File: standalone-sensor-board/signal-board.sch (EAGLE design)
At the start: 26 parts, among them U1 CD4051BE

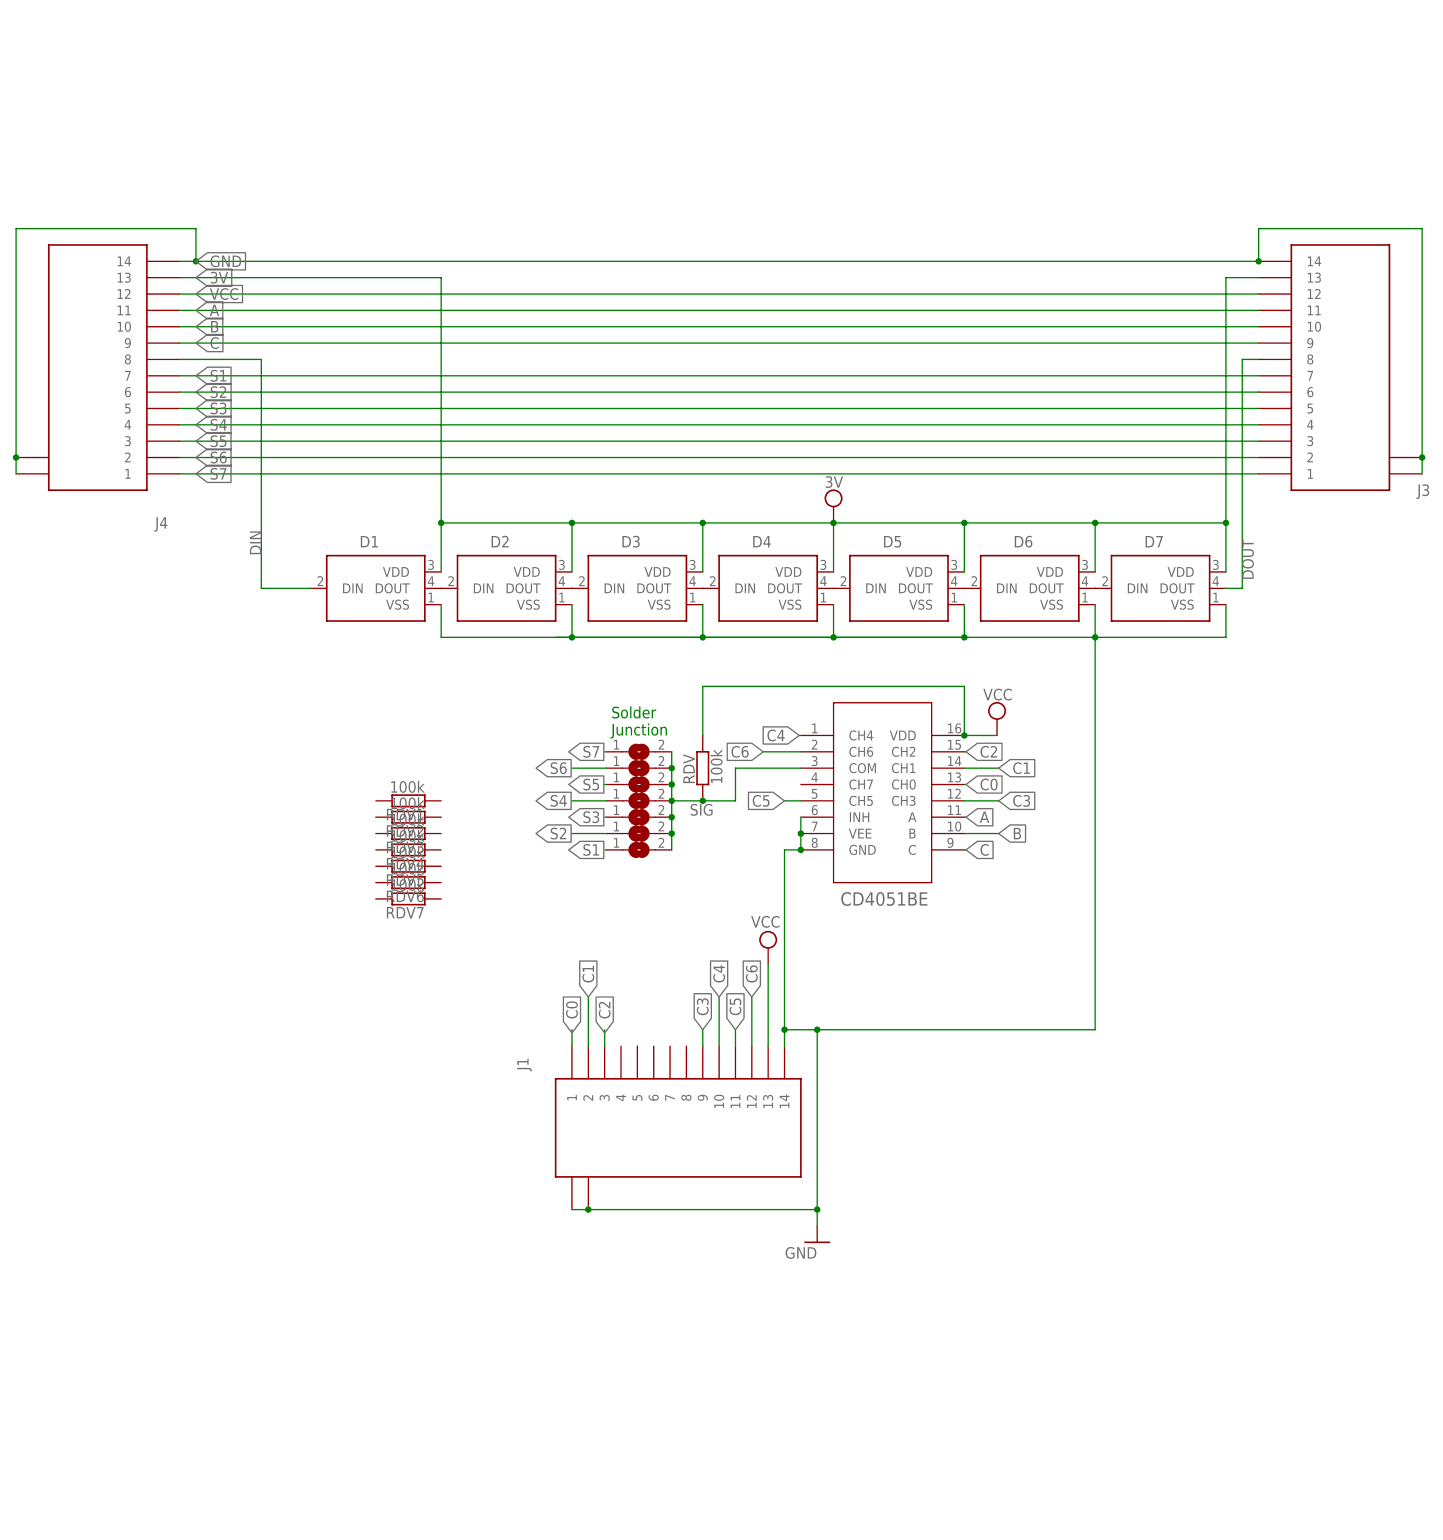
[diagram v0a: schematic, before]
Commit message: set rdvs
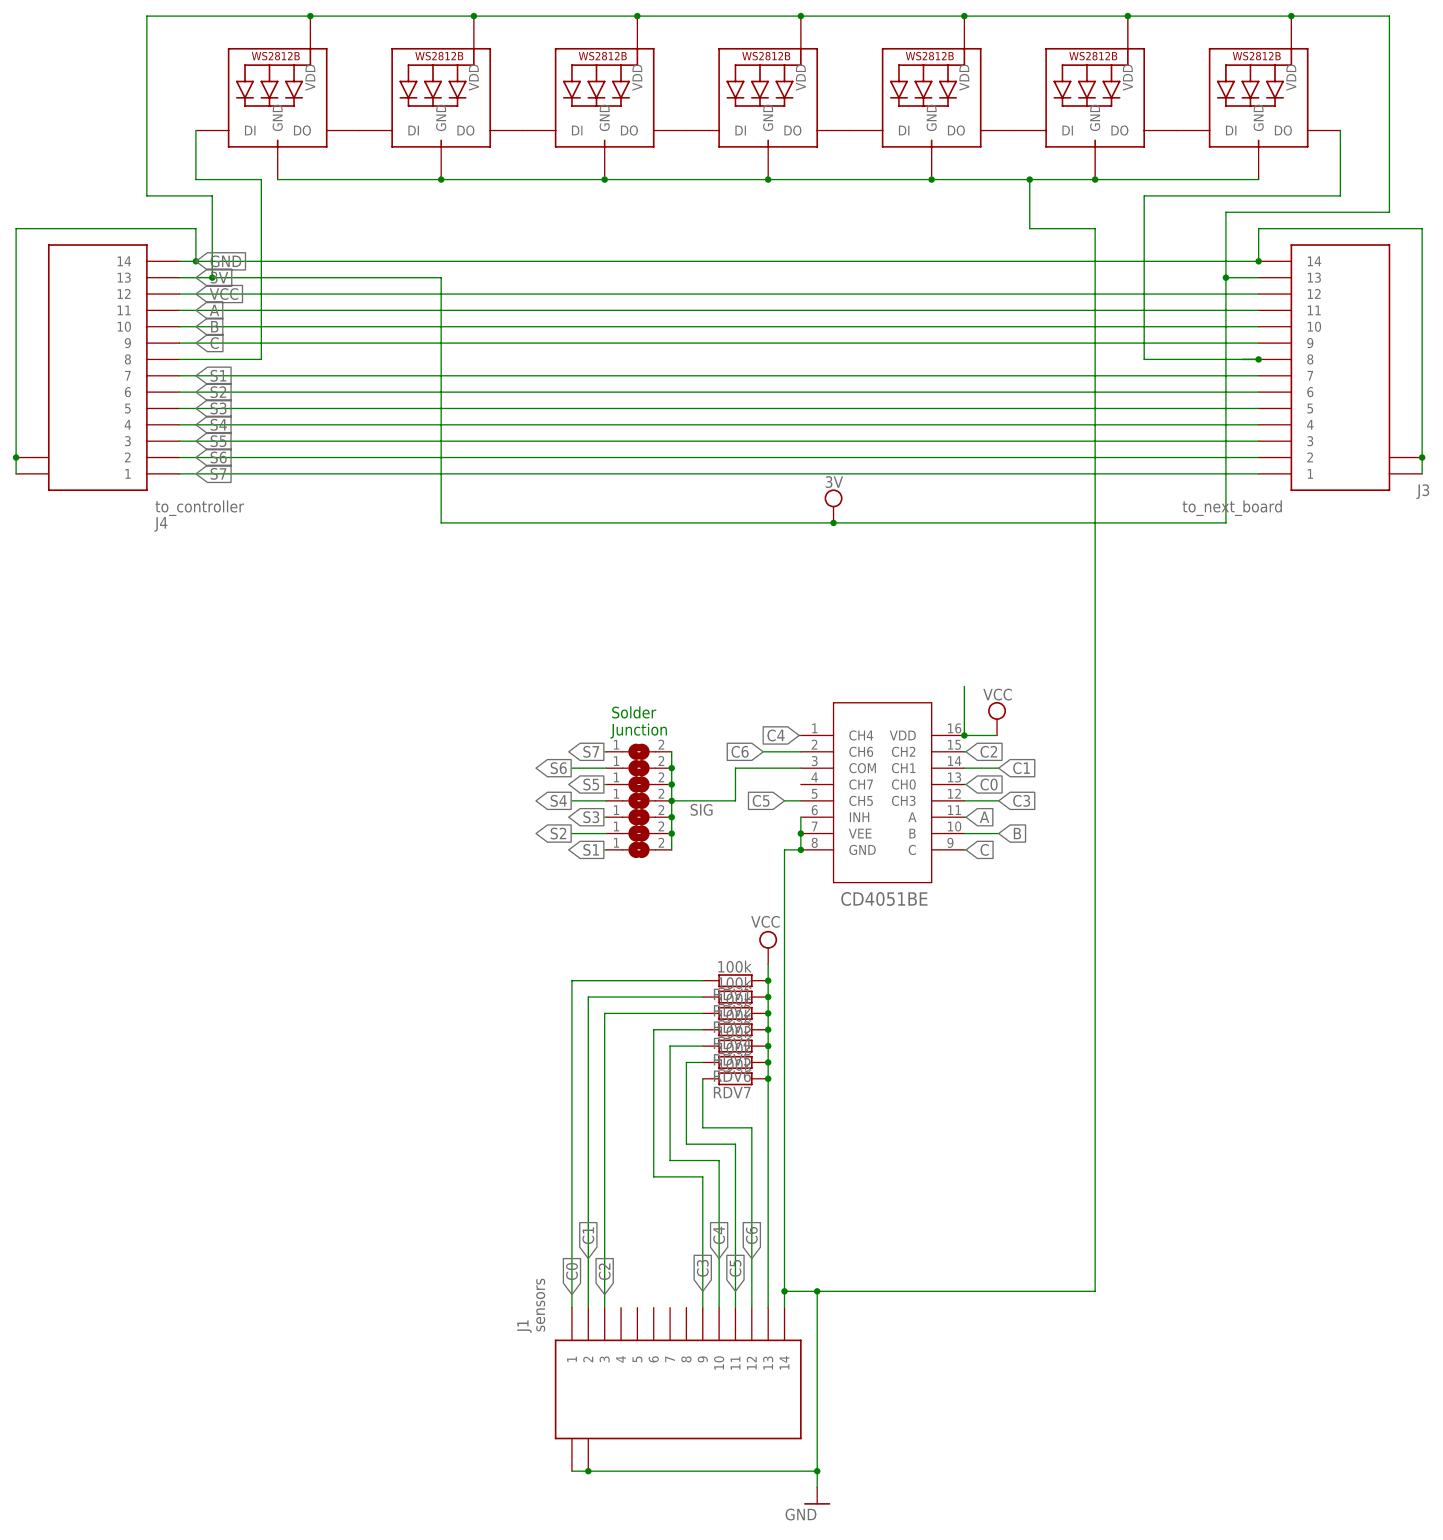
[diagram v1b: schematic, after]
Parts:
- removed D1, D2, D3, D4, D5, D6, D7: 1655, 1655:1655
- removed RDV: 100k, rcl:R-EU_0207/10
- added LED1, LED2, LED3, LED4, LED5, LED6, LED7: WS2812B3535, adafruit:WS2812B3535
- J1: value (none) -> sensors
- J3: value (none) -> to_next_board
- J4: value (none) -> to_controller
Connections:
- removed net N$15: D6.DOUT, D7.DIN
- removed net N$16: D1.DOUT, D2.DIN
- removed net N$17: D2.DOUT, D3.DIN
- removed net N$18: D3.DOUT, D4.DIN
- removed net N$19: D4.DOUT, D5.DIN
- removed net N$20: D5.DOUT, D6.DIN
- new net N$1: LED1.DO, LED2.DI
- new net N$2: LED2.DO, LED3.DI
- new net N$3: LED3.DO, LED4.DI
- new net N$4: LED4.DO, LED5.DI
- new net N$5: LED5.DO, LED6.DI
- new net N$6: LED6.DO, LED7.DI
- net 3V: now also LED1.VDD, LED2.VDD, LED3.VDD, LED4.VDD, LED5.VDD, LED6.VDD, LED7.VDD; no longer D1.VDD, D2.VDD, D3.VDD, D4.VDD, D5.VDD, D6.VDD, D7.VDD
- net C0: now also RDV1.2
- net C1: now also RDV2.2
- net C2: now also RDV3.2
- net C3: now also RDV4.2
- net C4: now also RDV5.2
- net C5: now also RDV6.2
- net C6: now also RDV7.2
- net DIN: now also LED1.DI; no longer D1.DIN
- net DOUT: now also LED7.DO; no longer D7.DOUT
- net GND: now also LED1.GND, LED2.GND, LED3.GND, LED4.GND, LED5.GND, LED6.GND, LED7.GND; no longer D1.VSS, D2.VSS, D3.VSS, D4.VSS, D5.VSS, D6.VSS, D7.VSS
- net SIG: no longer RDV.1
- net VCC: now also RDV1.1, RDV2.1, RDV3.1, RDV4.1, RDV5.1, RDV6.1, RDV7.1; no longer RDV.2
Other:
- moved on the sheet: J1, RDV1, RDV2, RDV3, RDV4, RDV5, RDV6, RDV7
